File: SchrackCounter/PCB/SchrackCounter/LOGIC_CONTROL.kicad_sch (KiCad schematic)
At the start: 2 parts

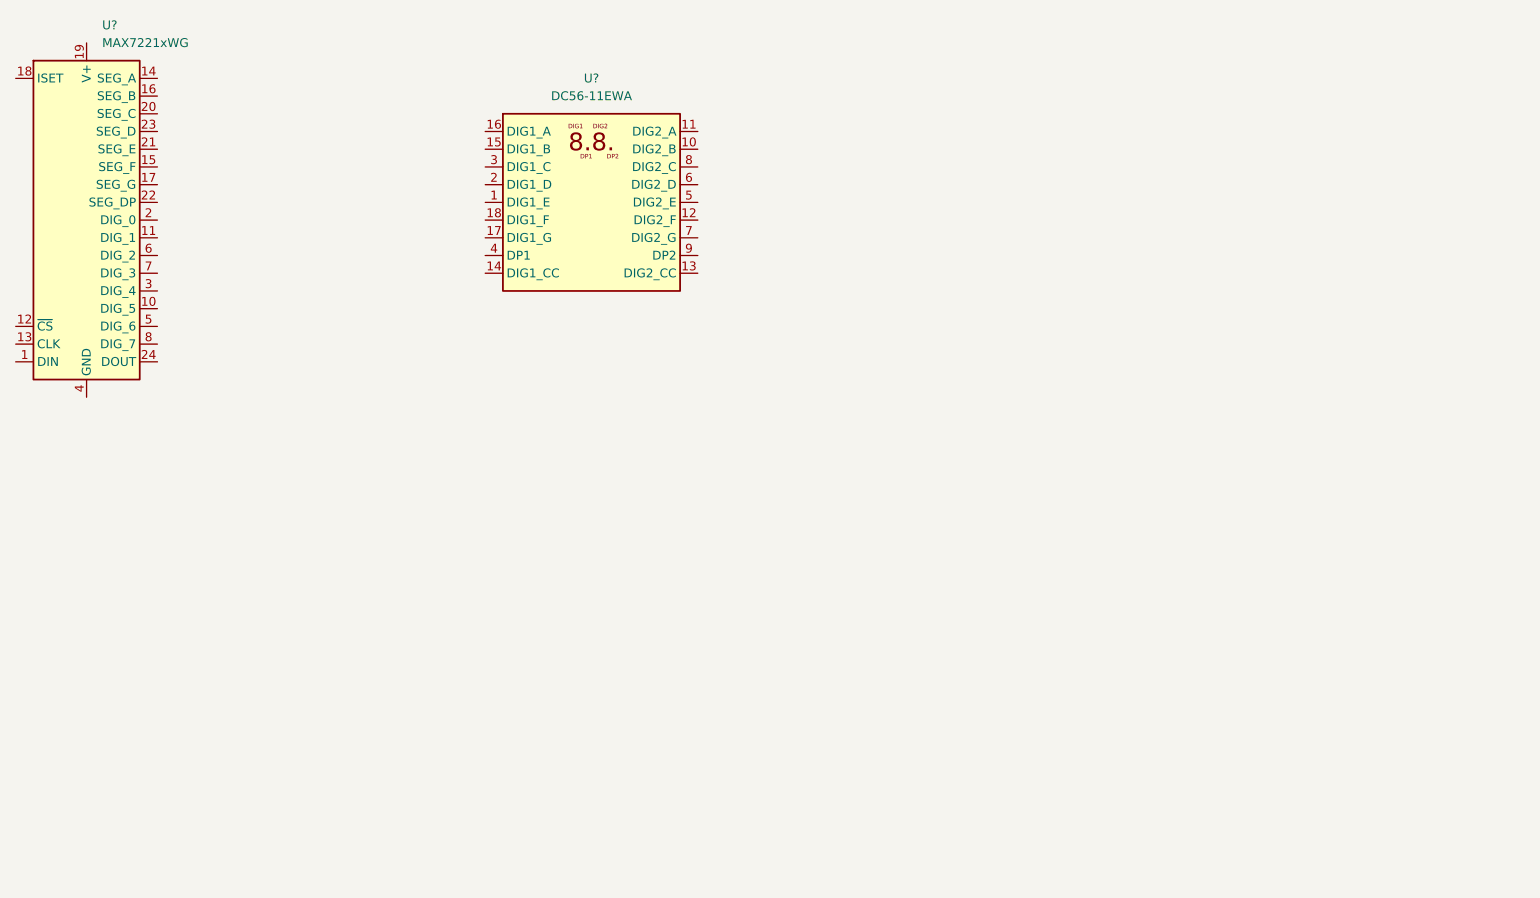
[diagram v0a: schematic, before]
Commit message: Schematic update
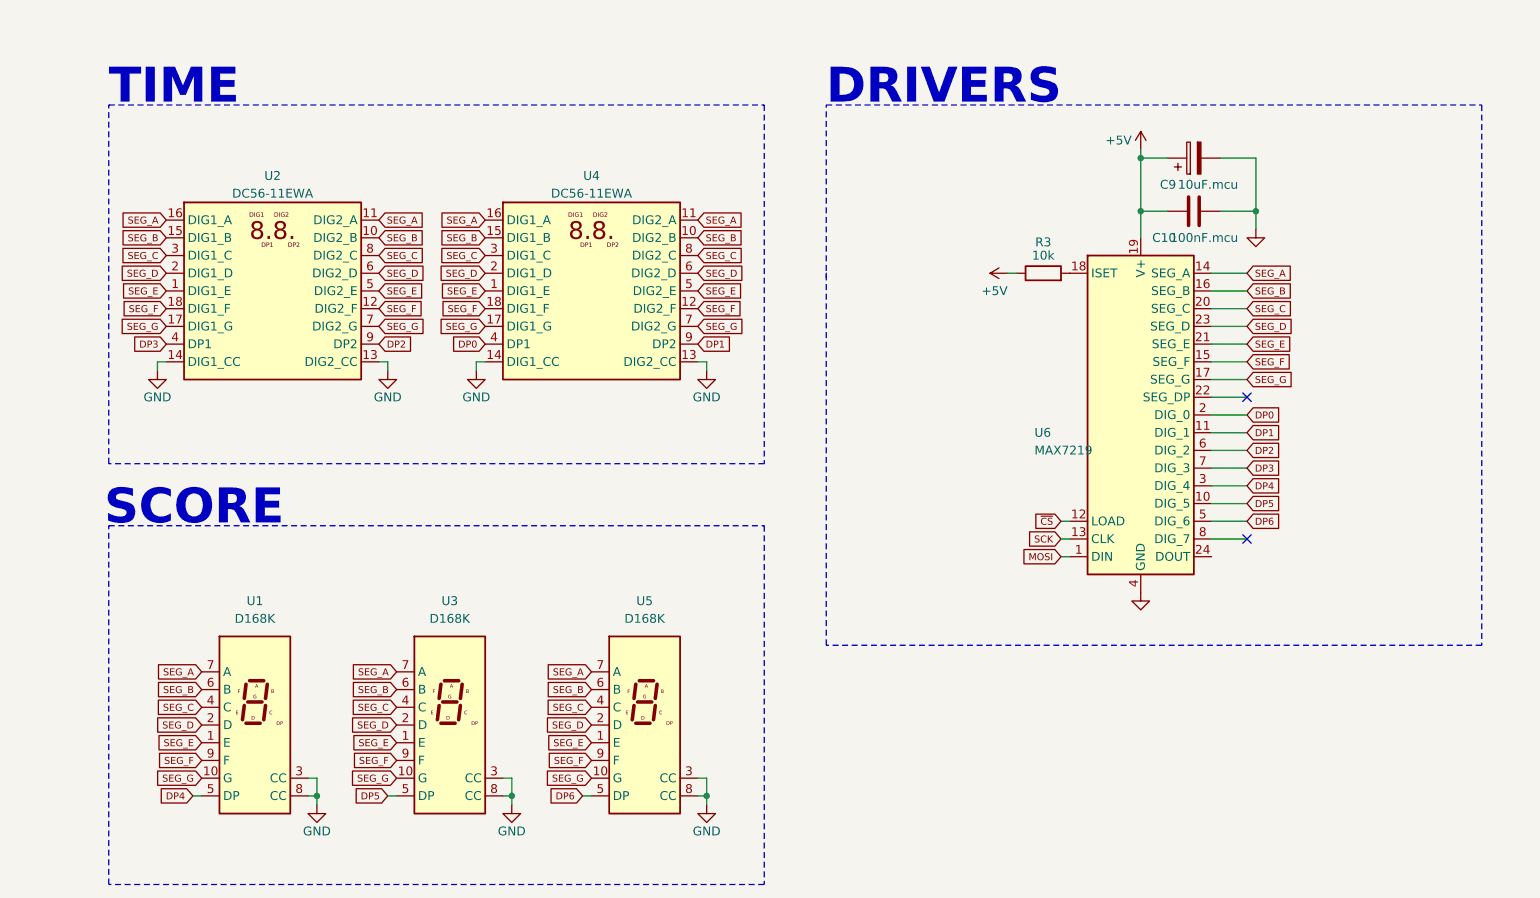
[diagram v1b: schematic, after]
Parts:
- removed U?: MAX7221xWG, Package_SO:SOIC-24W_7.5x15.4mm_P1.27mm, symbol Driver_LED:MAX7221xWG
- added C10: 100nF.mcu, Capacitor_SMD:C_0805_2012Metric_Pad1.18x1.45mm_HandSolder, symbol Device:C
- added C9: 10uF.mcu, Capacitor_Tantalum_SMD:CP_EIA-3216-18_Kemet-A_Pad1.58x1.35mm_HandSolder, symbol Device:C_Polarized
- added R3: 10k, symbol Device:R
- added U1, U3, U5: D168K, Display_7Segment:D1X8K, symbol Display_Character:D168K
- added U2: DC56-11EWA, Display_7Segment:DA56-11SURKWA, symbol Display_Character:DC56-11EWA
- added U6: MAX7219, symbol Driver_LED:MAX7219
- gave numbers to parts that had none: 1
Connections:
- net SEG_E: now reaches U4.1 (DIG1_E)
- net SEG_E: now also U4.5 (DIG2_E), U1.1 (E), U2.1 (DIG1_E), U2.5 (DIG2_E), U3.1 (E), U5.1 (E), U6.21 (SEG_E)
- net SEG_B: now reaches U4.10 (DIG2_B)
- net SEG_B: now also U4.15 (DIG1_B), U1.6 (B), U2.10 (DIG2_B), U2.15 (DIG1_B), U3.6 (B), U5.6 (B), U6.16 (SEG_B)
- net SEG_A: now reaches U4.11 (DIG2_A)
- net SEG_A: now also U4.16 (DIG1_A), U1.7 (A), U2.11 (DIG2_A), U2.16 (DIG1_A), U3.7 (A), U5.7 (A), U6.14 (SEG_A)
- net SEG_F: now reaches U4.12 (DIG2_F)
- net SEG_F: now also U4.18 (DIG1_F), U1.9 (F), U2.12 (DIG2_F), U2.18 (DIG1_F), U3.9 (F), U5.9 (F), U6.15 (SEG_F)
- net GND: now reaches U4.13 (DIG2_CC)
- net GND: now also U4.14 (DIG1_CC), C10.2, C9.2, U1.3 (CC), U1.8 (CC), U2.13 (DIG2_CC), U2.14 (DIG1_CC), U3.3 (CC), U3.8 (CC), U5.3 (CC), U5.8 (CC), U6.4 (GND), U6.9 (GND)
- net SEG_G: now reaches U4.17 (DIG1_G)
- net SEG_G: now also U4.7 (DIG2_G), U1.10 (G), U2.17 (DIG1_G), U2.7 (DIG2_G), U3.10 (G), U5.10 (G), U6.17 (SEG_G)
- net SEG_D: now reaches U4.2 (DIG1_D)
- net SEG_D: now also U4.6 (DIG2_D), U1.2 (D), U2.2 (DIG1_D), U2.6 (DIG2_D), U3.2 (D), U5.2 (D), U6.23 (SEG_D)
- net SEG_C: now reaches U4.3 (DIG1_C)
- net SEG_C: now also U4.8 (DIG2_C), U1.4 (C), U2.3 (DIG1_C), U2.8 (DIG2_C), U3.4 (C), U5.4 (C), U6.20 (SEG_C)
- net DP0: now reaches U4.4 (DP1)
- net DP0: now also U6.2 (DIG_0)
- net DP1: now reaches U4.9 (DP2)
- net DP1: now also U6.11 (DIG_1)
- new net: R3.2, U6.18 (ISET)
- new net +5V: C10.1, C9.1, R3.1, U6.19 (V+)
- new net DP2: U2.9 (DP2), U6.6 (DIG_2)
- new net DP3: U2.4 (DP1), U6.7 (DIG_3)
- new net DP4: U1.5 (DP), U6.3 (DIG_4)
- new net DP5: U3.5 (DP), U6.10 (DIG_5)
- new net DP6: U5.5 (DP), U6.5 (DIG_6)
- new net MOSI: U6.1 (DIN)
- new net SCK: U6.13 (CLK)
- new net ~{CS}: U6.12 (LOAD)
- no-connect marks 0 -> 2
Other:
- note added: "DRIVERS"
- note added: "SCORE"
- note added: "TIME"
- moved on the sheet: U4

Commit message: Schematic update
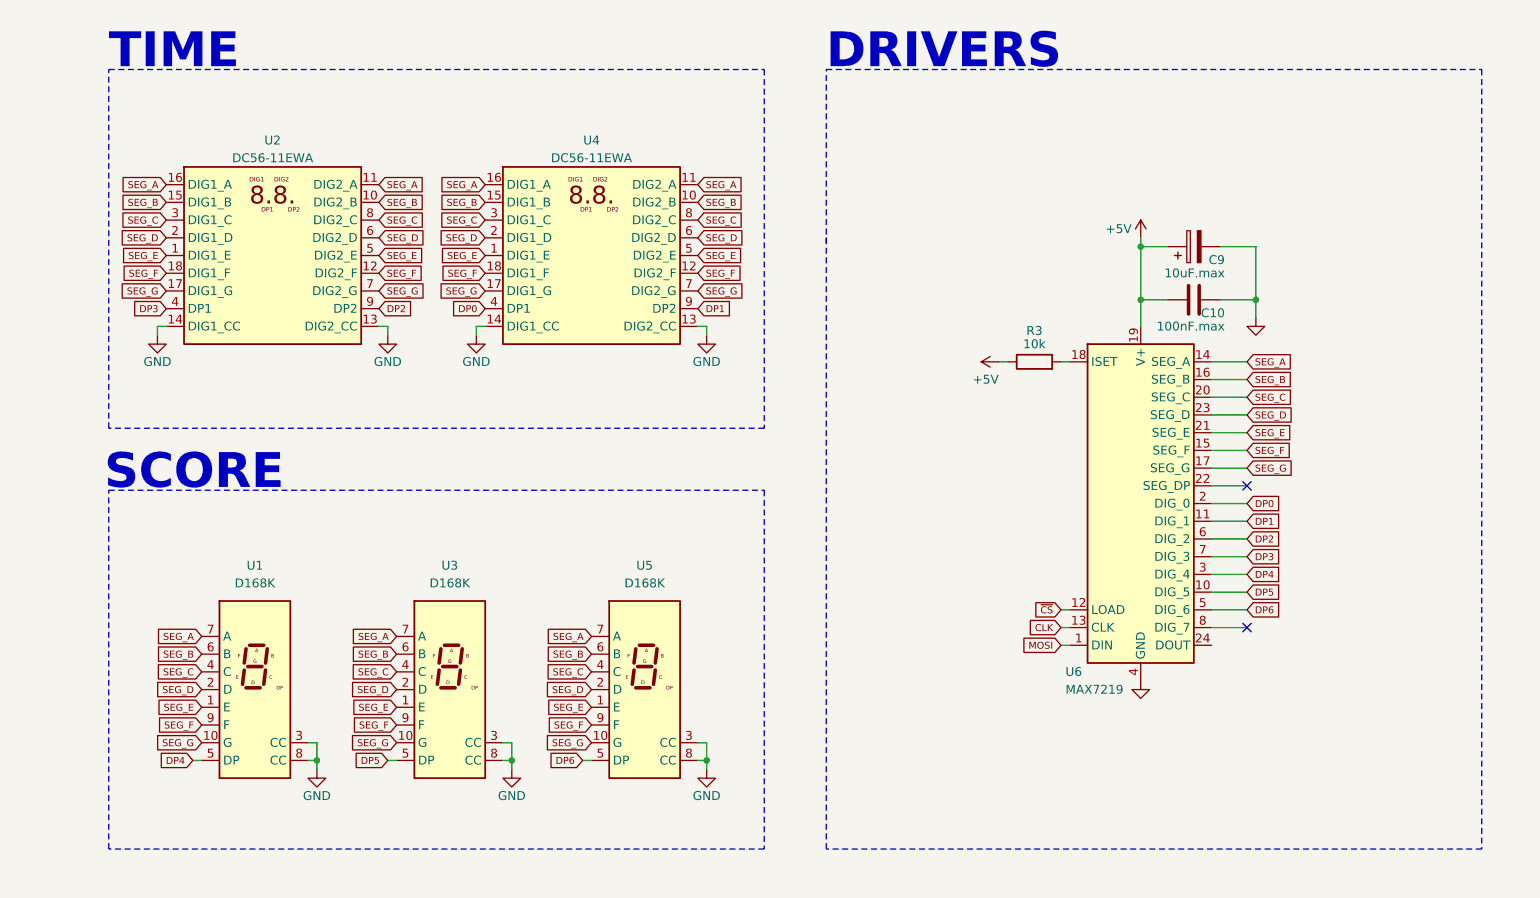
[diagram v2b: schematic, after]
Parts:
- C10: value 100nF.mcu -> 100nF.max
- C9: value 10uF.mcu -> 10uF.max
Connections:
- net SCK renamed CLK
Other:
- moved on the sheet: C10, C9, R3, U1, U2, U3, U4, U5, U6

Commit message: sleep, overated imo
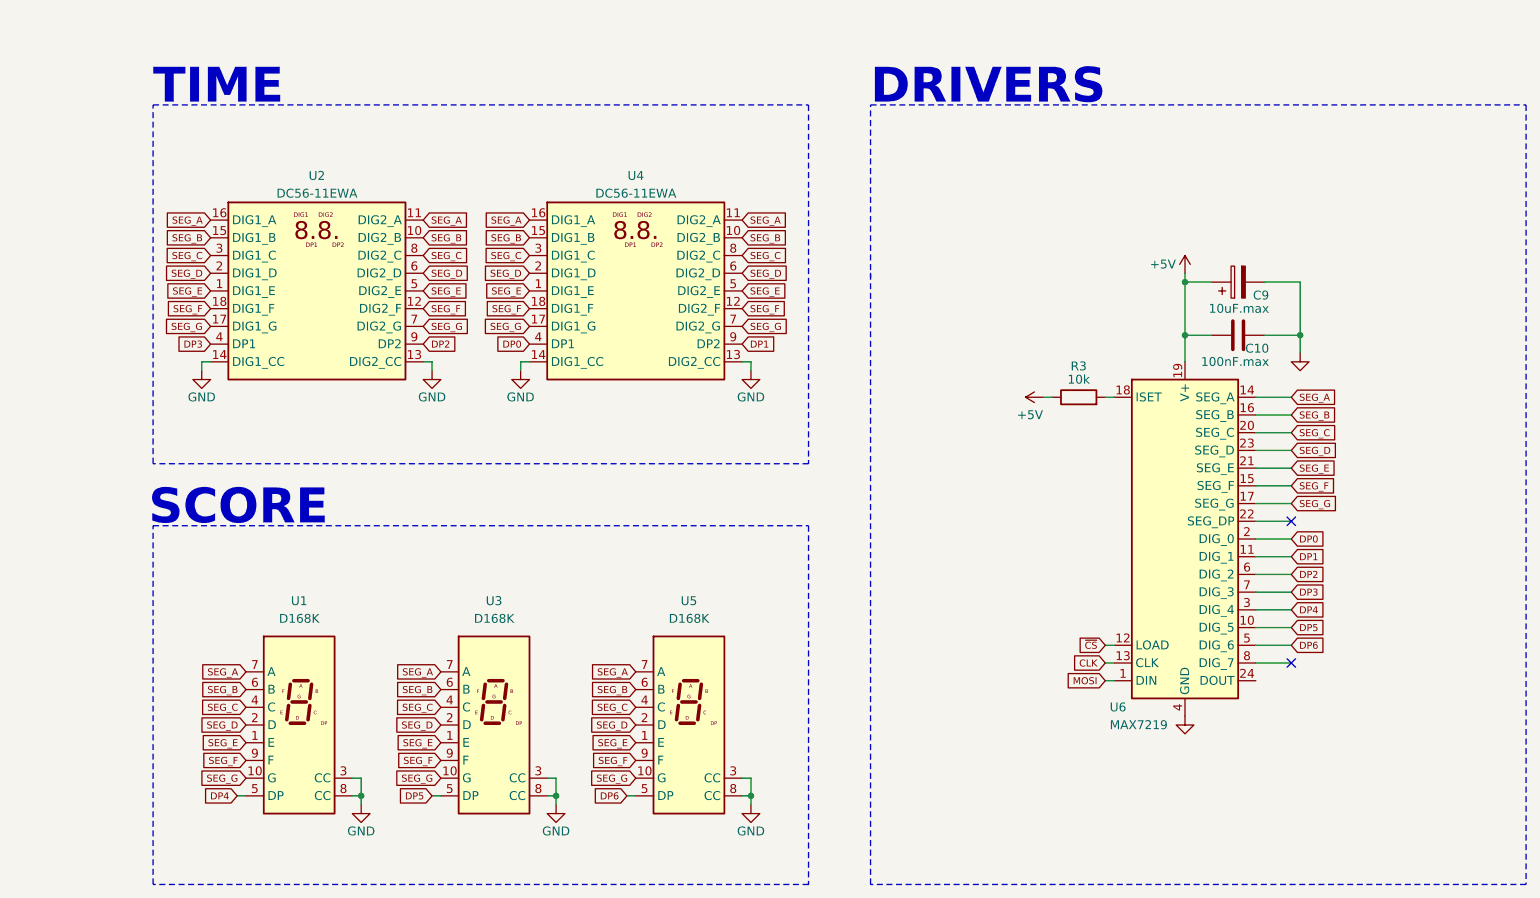
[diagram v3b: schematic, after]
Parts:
- R3: footprint (none) -> Resistor_SMD:R_0805_2012Metric_Pad1.20x1.40mm_HandSolder
- U6: footprint (none) -> Package_SO:SOIC-24W_7.5x15.4mm_P1.27mm
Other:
- moved on the sheet: C10, C9, R3, U1, U2, U3, U4, U5, U6
